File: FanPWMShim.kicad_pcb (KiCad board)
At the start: 2 copper layers, 53.3 x 14 mm, 5 parts, among them J1 Raspberry_Pi_2_3, J2 Conn_01x02_Female, Q1 MMBT2222A

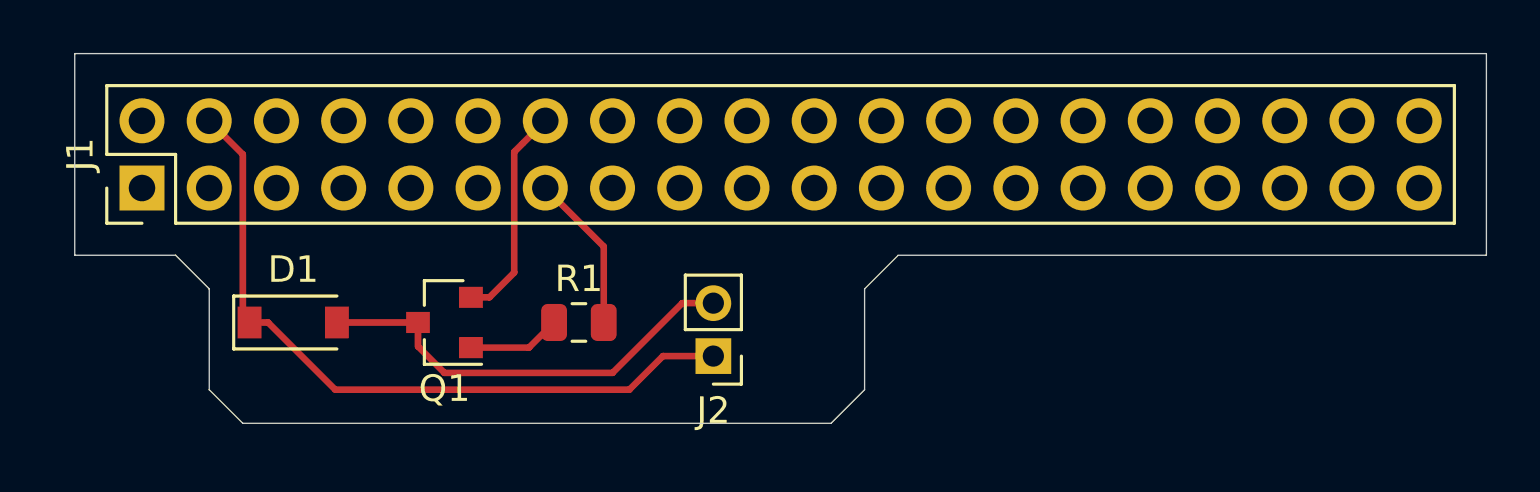
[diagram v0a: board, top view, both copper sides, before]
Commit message: Update PCB
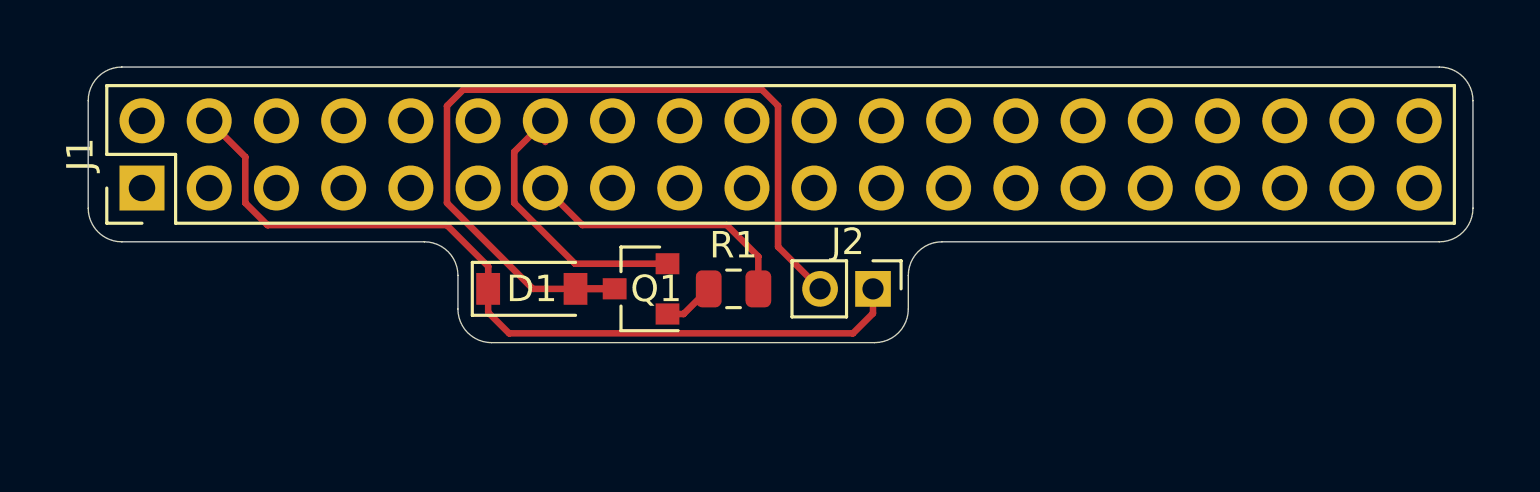
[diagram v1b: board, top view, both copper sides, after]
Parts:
- moved D1 9.11 mm to (30.0, 21.6)
- moved Q1 7.54 mm to (34.1, 21.6)
- moved J2 6.55 mm to (42.9, 21.6), turned to 270 degrees
- moved R1 5.98 mm to (37.6, 21.6)
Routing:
- net Net-(D1-Pad2): track 17.0 -> 33.4 mm
- net Net-(J1-Pad13): track 5.99 -> 10.4 mm
- net Net-(D1-Pad1): track 27.7 -> 31.7 mm
- net Net-(J1-Pad14): track 8.24 -> 11.1 mm
- net Net-(Q1-Pad1): track 3.54 -> 1.95 mm
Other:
- board size 53.3 x 14 mm -> 52.3 x 10.4 mm
- board text added: "pwm fan shim d0pefish 2019"
